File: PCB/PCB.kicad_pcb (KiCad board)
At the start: 2 copper layers, 95 x 62.5 mm, 19 parts, among them J1 Conn_01x04_Pin, J2 Conn_01x05_Pin, J3 Conn_01x04_Pin, SW1 SW_SPDT, SW2 SW_Push, U1 ESP32-DevKitC

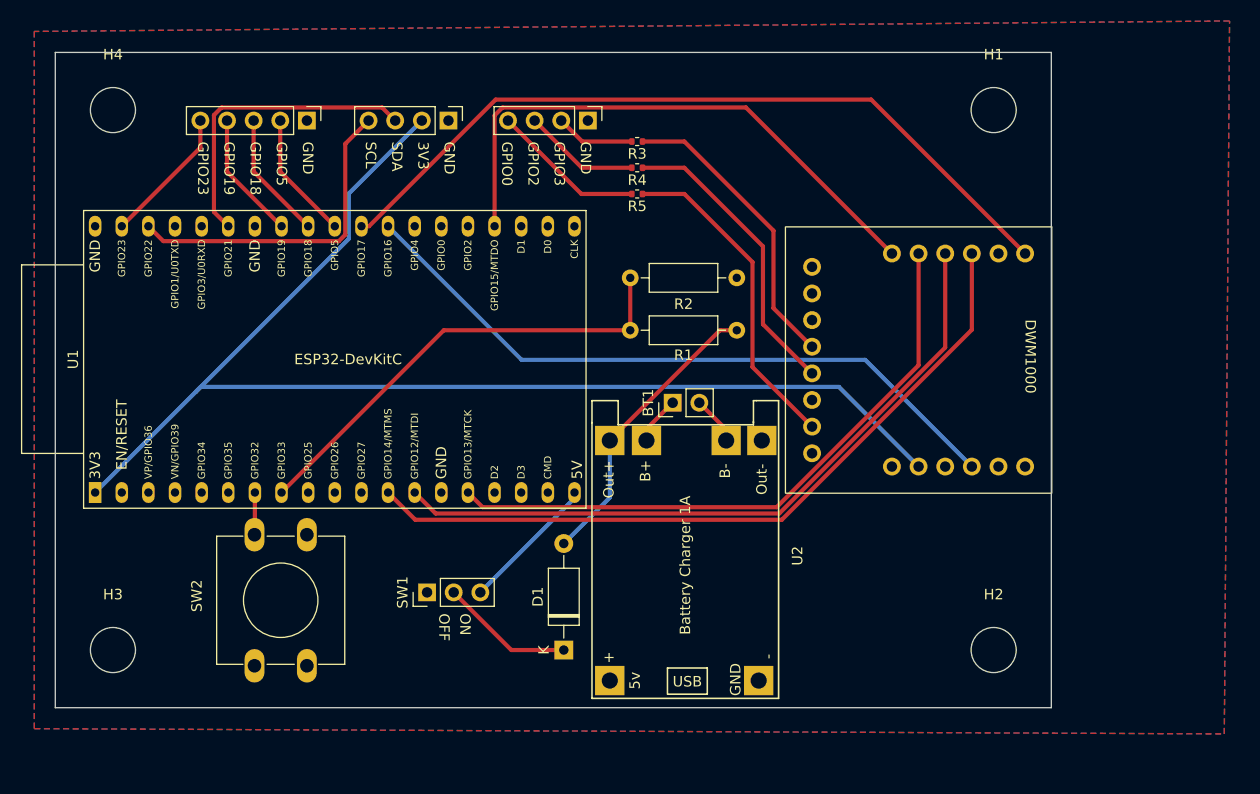
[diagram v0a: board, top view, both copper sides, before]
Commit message: PCB redesign
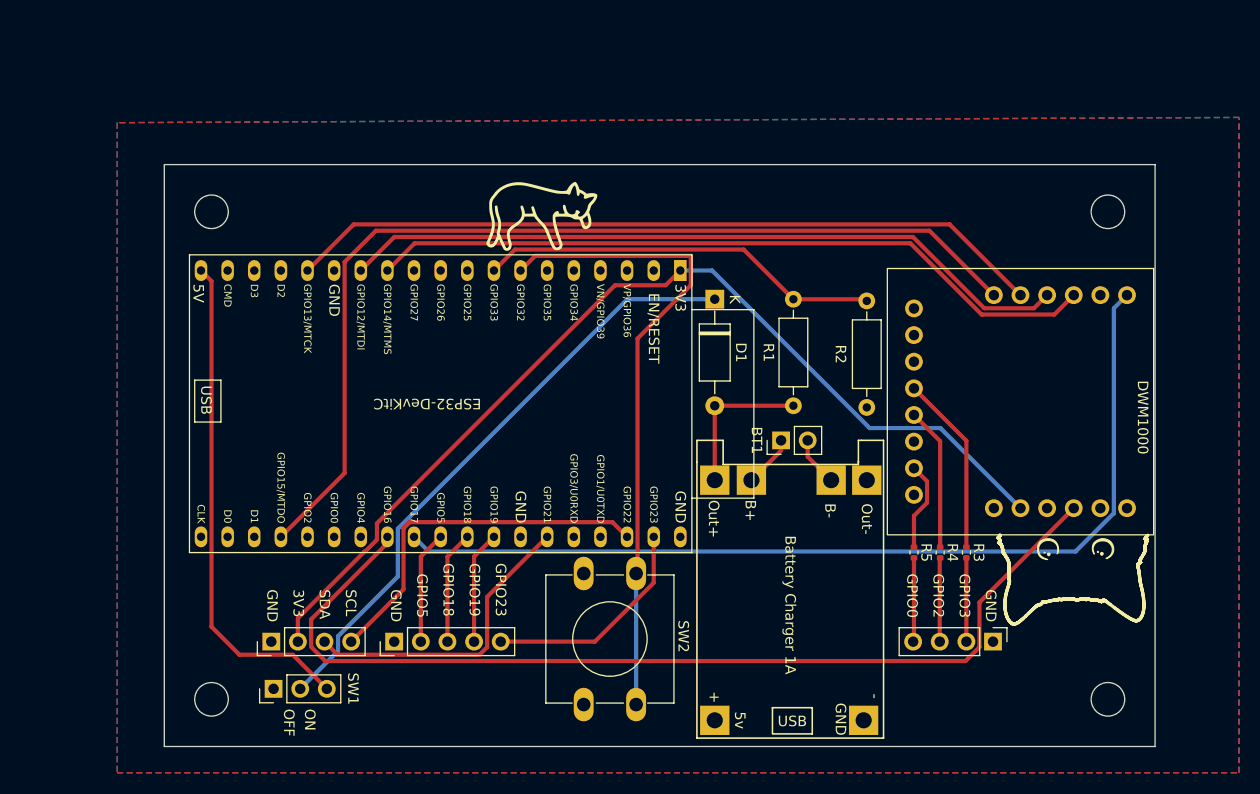
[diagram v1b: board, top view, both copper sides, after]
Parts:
- H1, H2, H3, H4: footprint MountingHole:MountingHole_4.3mm_M4 -> MountingHole:MountingHole_3.2mm_M3
- moved H3 95.0 mm to (144.9, 113.7)
- moved H1 75.2 mm to (59.4, 67.2)
- moved J3 63.0 mm to (133.9, 108.2)
- moved U1 59.7 mm to (104.1, 72.8), turned to -90 degrees
- moved H4 57.0 mm to (59.4, 113.7)
- moved J1 52.5 mm to (65.1, 108.2), turned to 90 degrees
- moved J2 50.4 mm to (76.8, 108.2), turned to 90 degrees
- moved R3 50.2 mm to (131.4, 99.7), turned to -90 degrees
- moved R4 46.7 mm to (128.9, 99.7), turned to -90 degrees
- moved R5 43.2 mm to (126.4, 99.7), turned to -90 degrees
- moved H2 43.2 mm to (144.9, 67.2)
- moved D1 36.4 mm to (107.4, 75.5), turned to -90 degrees
- moved SW2 31.0 mm to (94.9, 114.2), turned to 90 degrees
- moved R2 22.7 mm to (121.9, 75.7), turned to -90 degrees
- moved SW1 17.3 mm to (65.3, 112.7)
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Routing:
- net Net-(U1-32K_XP/GPIO32/ADC1_CH4): track 4.04 -> 61.8 mm
- net +5V: track 12.8 -> 58.4 mm
- net /CS: track 54.5 -> 94.4 mm
- net Net-(SW1-C): track 13.2 -> 47.8 mm
- net /RST: track 65.2 -> 95.3 mm
- net +3.3V: track 120.7 -> 95.2 mm
- net Net-(DWM1000-GPIO0): track 31.2 -> 8.57 mm
- net /IRQ: track 74.4 -> 90.2 mm
- net Net-(DWM1000-GPIO2): track 28.6 -> 13.6 mm
- net Net-(D1-A): track 28.1 -> 14.6 mm
- net /MOSI: track 59.8 -> 72.6 mm
- net Net-(DWM1000-GPIO3): track 28.6 -> 17.2 mm
- net /GPIO23: track 13.2 -> 21.3 mm
- net Net-(J3-Pin_4): track 14.7 -> 8.02 mm
- net VBAT: track 44.7 -> 38.4 mm
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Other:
- board size 95 x 62.5 mm -> 94.5 x 55.5 mm
- board text added: "USB"
